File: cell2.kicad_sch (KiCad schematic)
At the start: 26 parts, among them K1 V23105A5001A201, Q1 IRLML0030, Q2 IRLML0030, SW4 SW_SPST, SW5 SW_SPST

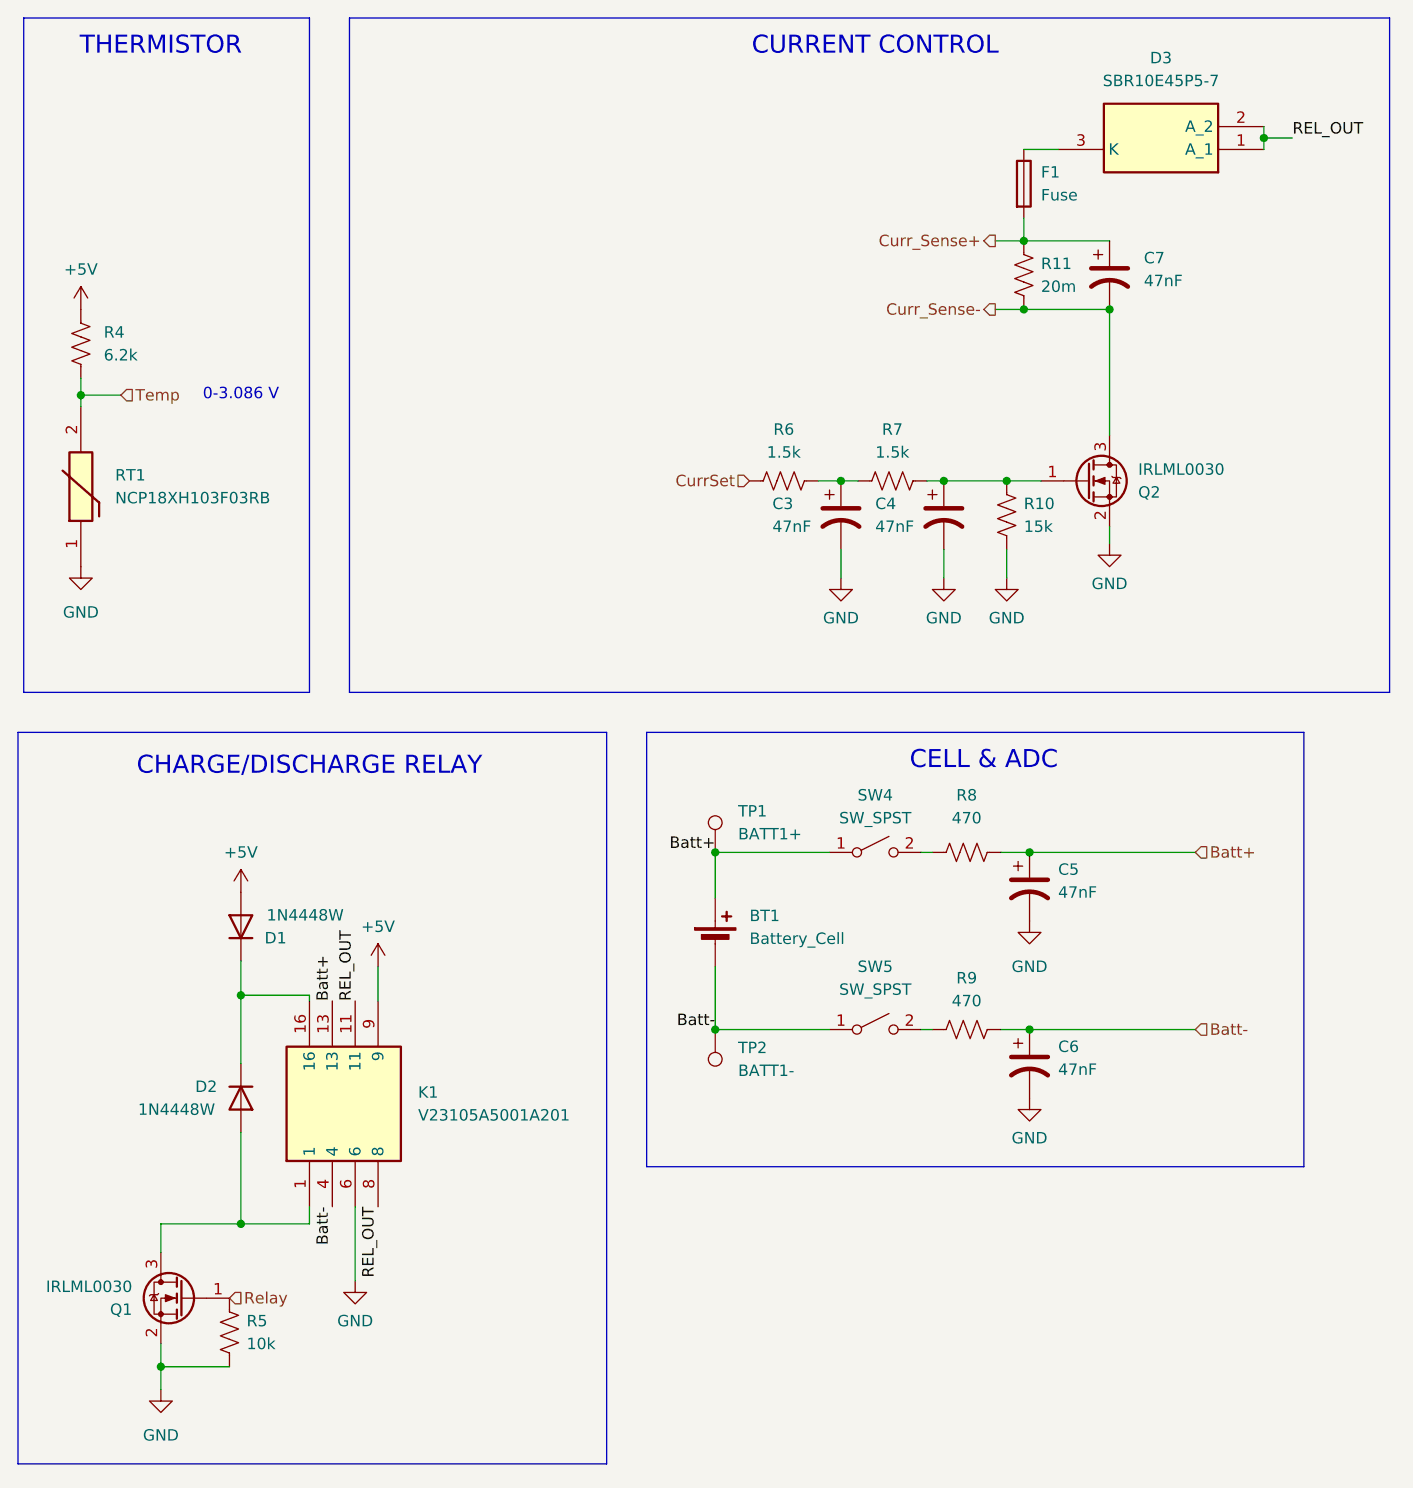
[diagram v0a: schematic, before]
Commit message: All footprints assigned
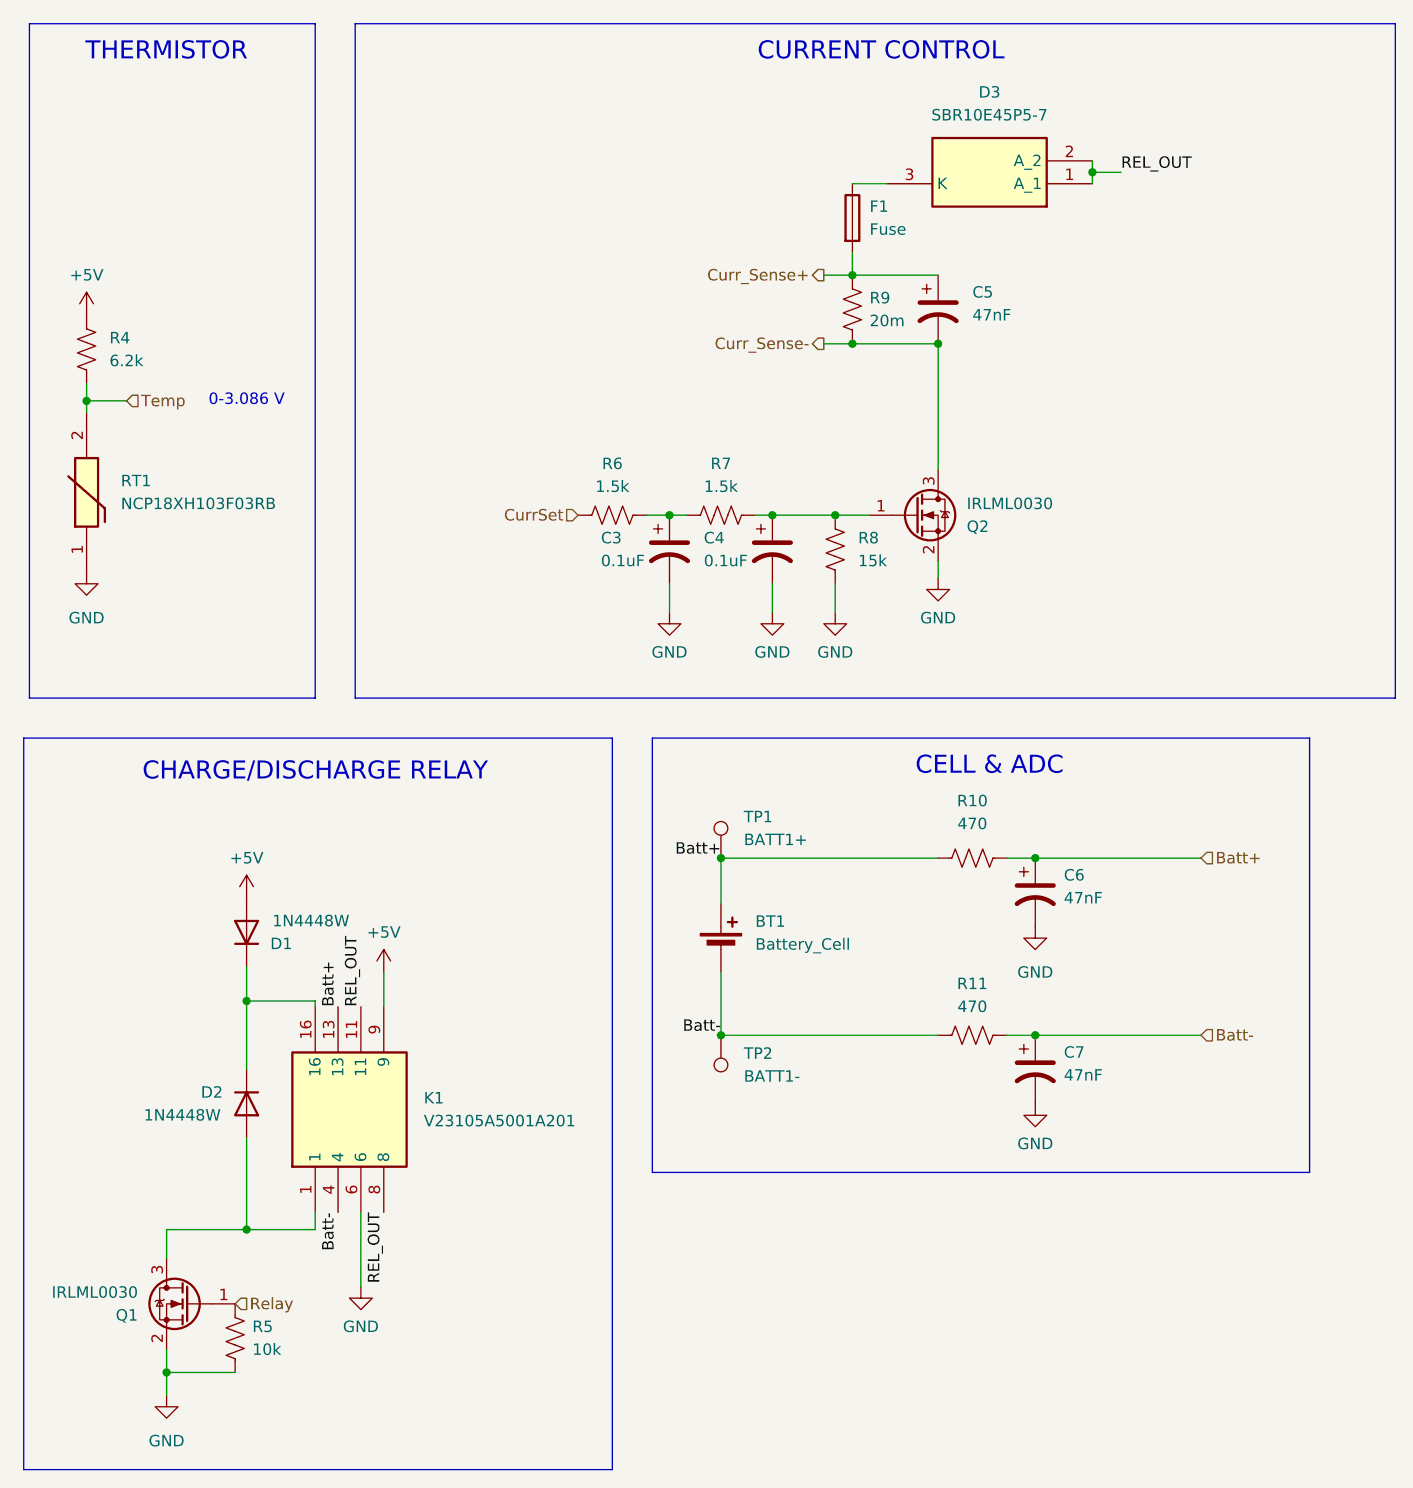
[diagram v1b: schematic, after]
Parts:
- removed SW4, SW5: SW_SPST, symbol Switch:SW_SPST
- C3, C4: value 47nF -> 0.1uF; footprint (none) -> Capacitor_SMD:C_0805_2012Metric
- C5, C6, C7: footprint (none) -> Capacitor_SMD:C_0805_2012Metric
- F1: footprint (none) -> Fuse:Fuse_1812_4532Metric
- R10: value 15k -> 470; footprint (none) -> Resistor_SMD:R_0805_2012Metric
- R11: value 20m -> 470; footprint (none) -> Resistor_SMD:R_0805_2012Metric
- R4, R5, R6, R7: footprint (none) -> Resistor_SMD:R_0805_2012Metric
- R8: value 470 -> 15k; footprint (none) -> Resistor_SMD:R_0805_2012Metric
- R9: value 470 -> 20m; footprint (none) -> Resistor_SMD:R_1206_3216Metric
- TP1, TP2: footprint (none) -> UTSVT_Special:TestPoint_HEX_3mmID
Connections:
- net Batt+: now also C6.1, R10.1, R10.2; no longer C5.1, R8.2
- net Batt-: now also C7.1, R11.1, R11.2; no longer C6.1, R9.2
- net Curr_Sense+: now also C5.1, R9.1; no longer C7.1, R11.1
- net Curr_Sense-: now also C5.2, R9.2; no longer C7.2, R11.2
- net GND: now also C7.2, R8.1; no longer C5.2, R10.1
- net at C4.1, Q2.1 (G), R7.2: now also R8.2; no longer R10.2
